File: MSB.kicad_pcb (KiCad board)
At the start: 2 copper layers, 39.1 x 40.6 mm, 26 parts, among them J1 22-05-3021, J2 22-05-3021, J3 90120-0763, J4 90120-0763, J5 22-05-3021, P1 22-27-2041, P2 22-27-2041, P3 61300811121, Q1 FDN5632N-F085, Q2 FDN5632N-F085, U1 MSP430FR2355TPTR, U2 LD1117S33TR

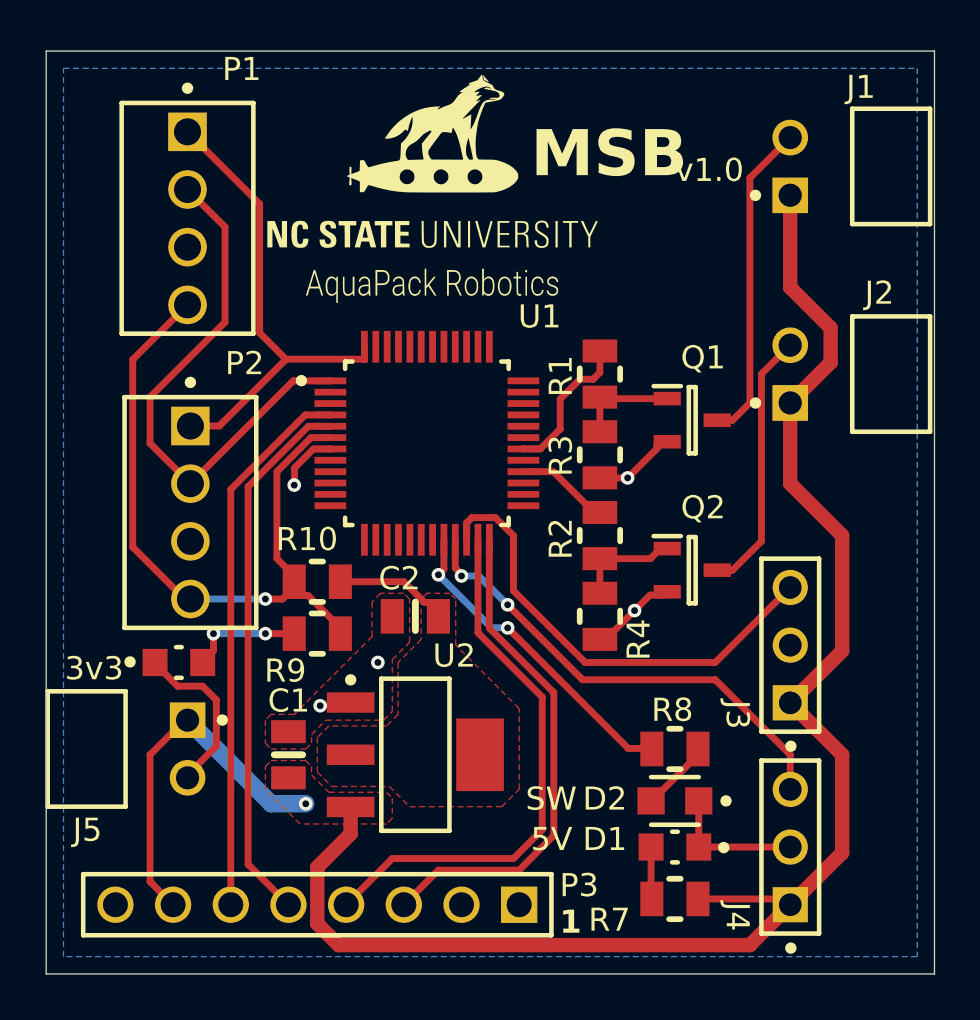
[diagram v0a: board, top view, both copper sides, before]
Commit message: v2
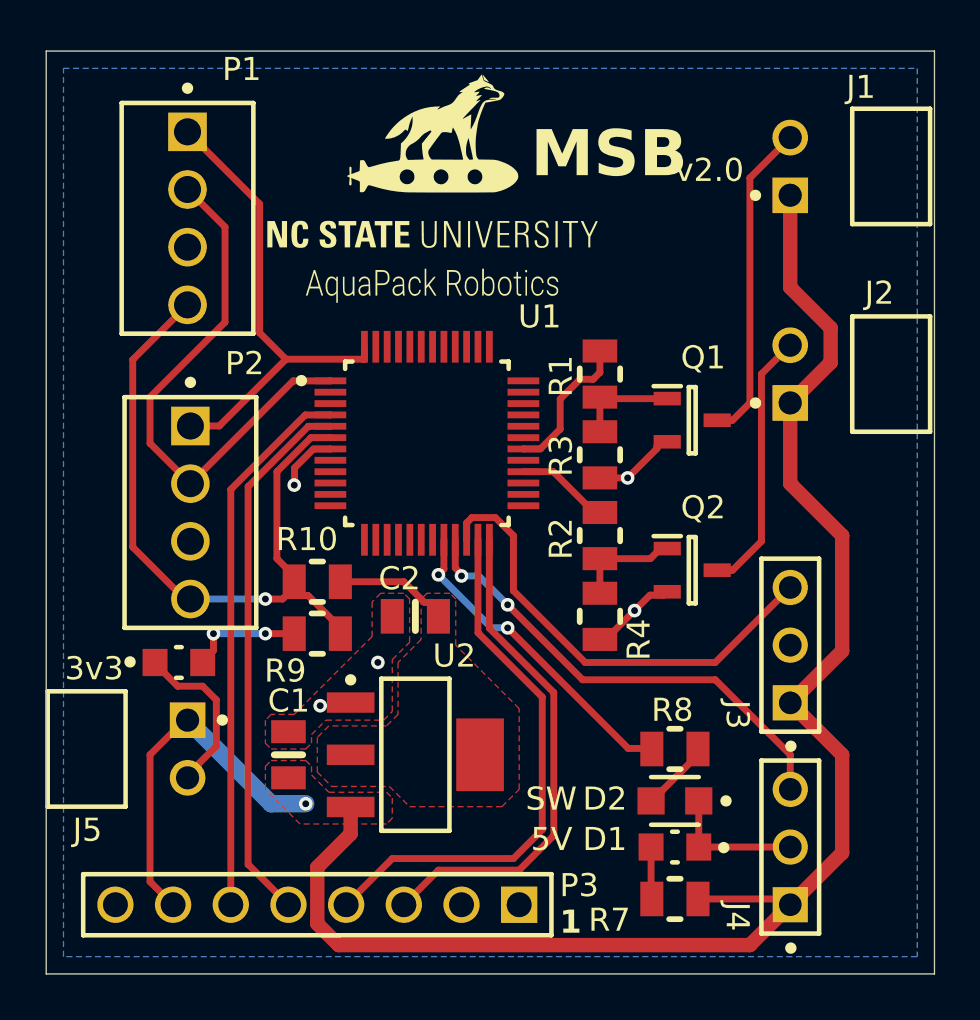
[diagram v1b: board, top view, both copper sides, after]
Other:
- board text added: "v2.0"
- board text removed: "v1.0"

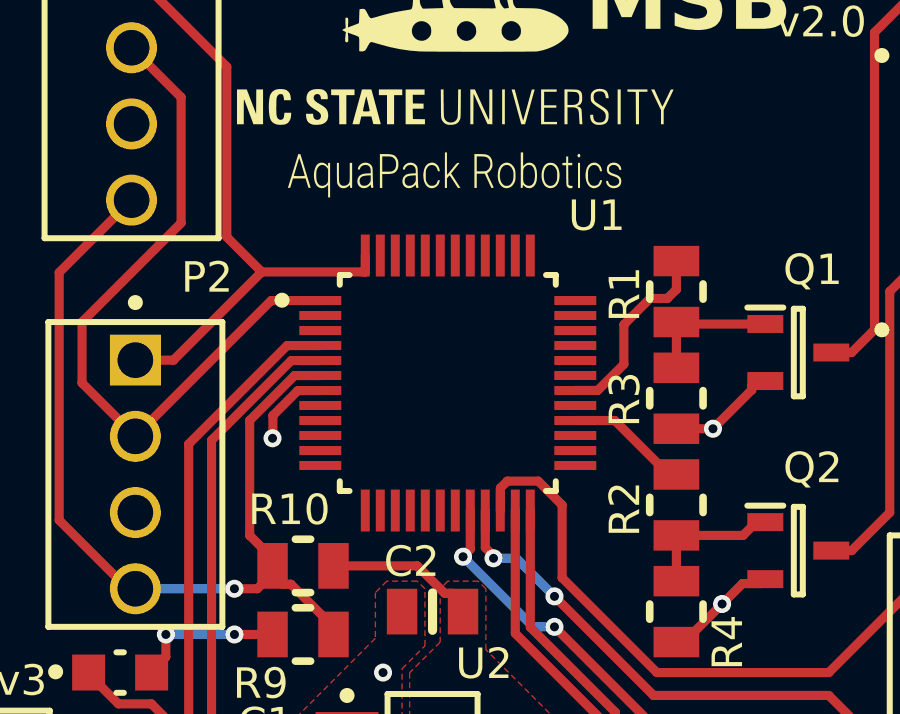
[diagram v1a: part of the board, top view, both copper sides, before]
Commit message: Update STM32
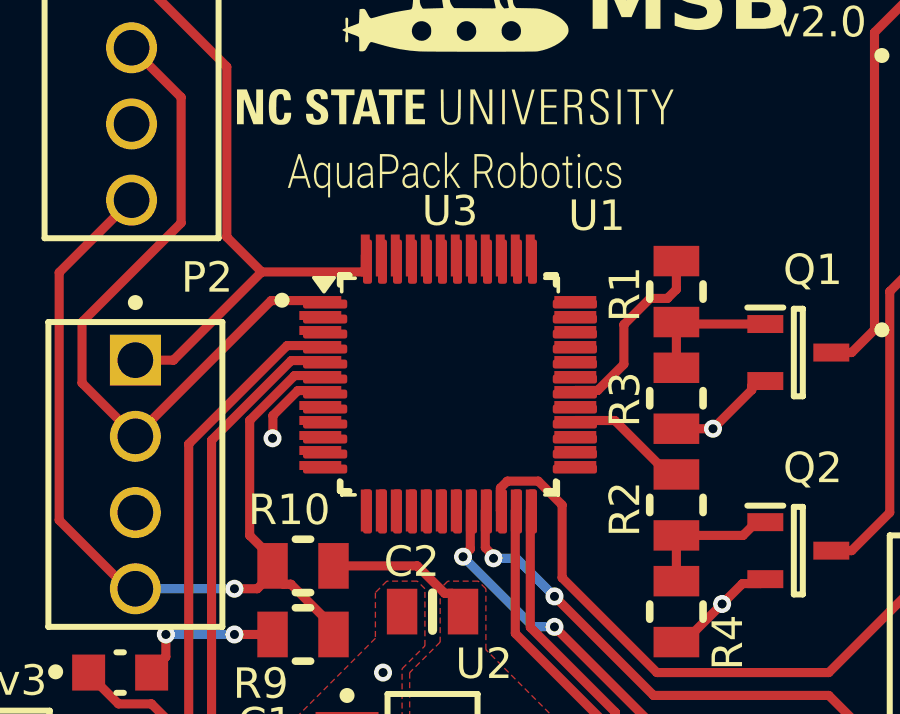
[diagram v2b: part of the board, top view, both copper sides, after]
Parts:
- added U3: STM32L051C6Tx, Package_QFP:LQFP-48_7x7mm_P0.5mm, F.Cu at (145.8, 102.1)
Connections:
- J3 pad 3: /SERVO1_CTRL -> +5
- P3 pad 3: /RXD -> unconnected-(P3-Pad3)
- P3 pad 4: /TXD -> +5
- P3 pad 5: /RST -> unconnected-(P3-Pad5)
- P3 pad 6: /TST -> unconnected-(P3-Pad6)
- R8 pad 1: Net-(U1-P6.2/TB3.3) -> unconnected-(R8-Pad1)
